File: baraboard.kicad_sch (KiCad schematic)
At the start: 27 parts, among them J1 OLED_128x64, U1 MCU_Seeed_XIAO_RP2040

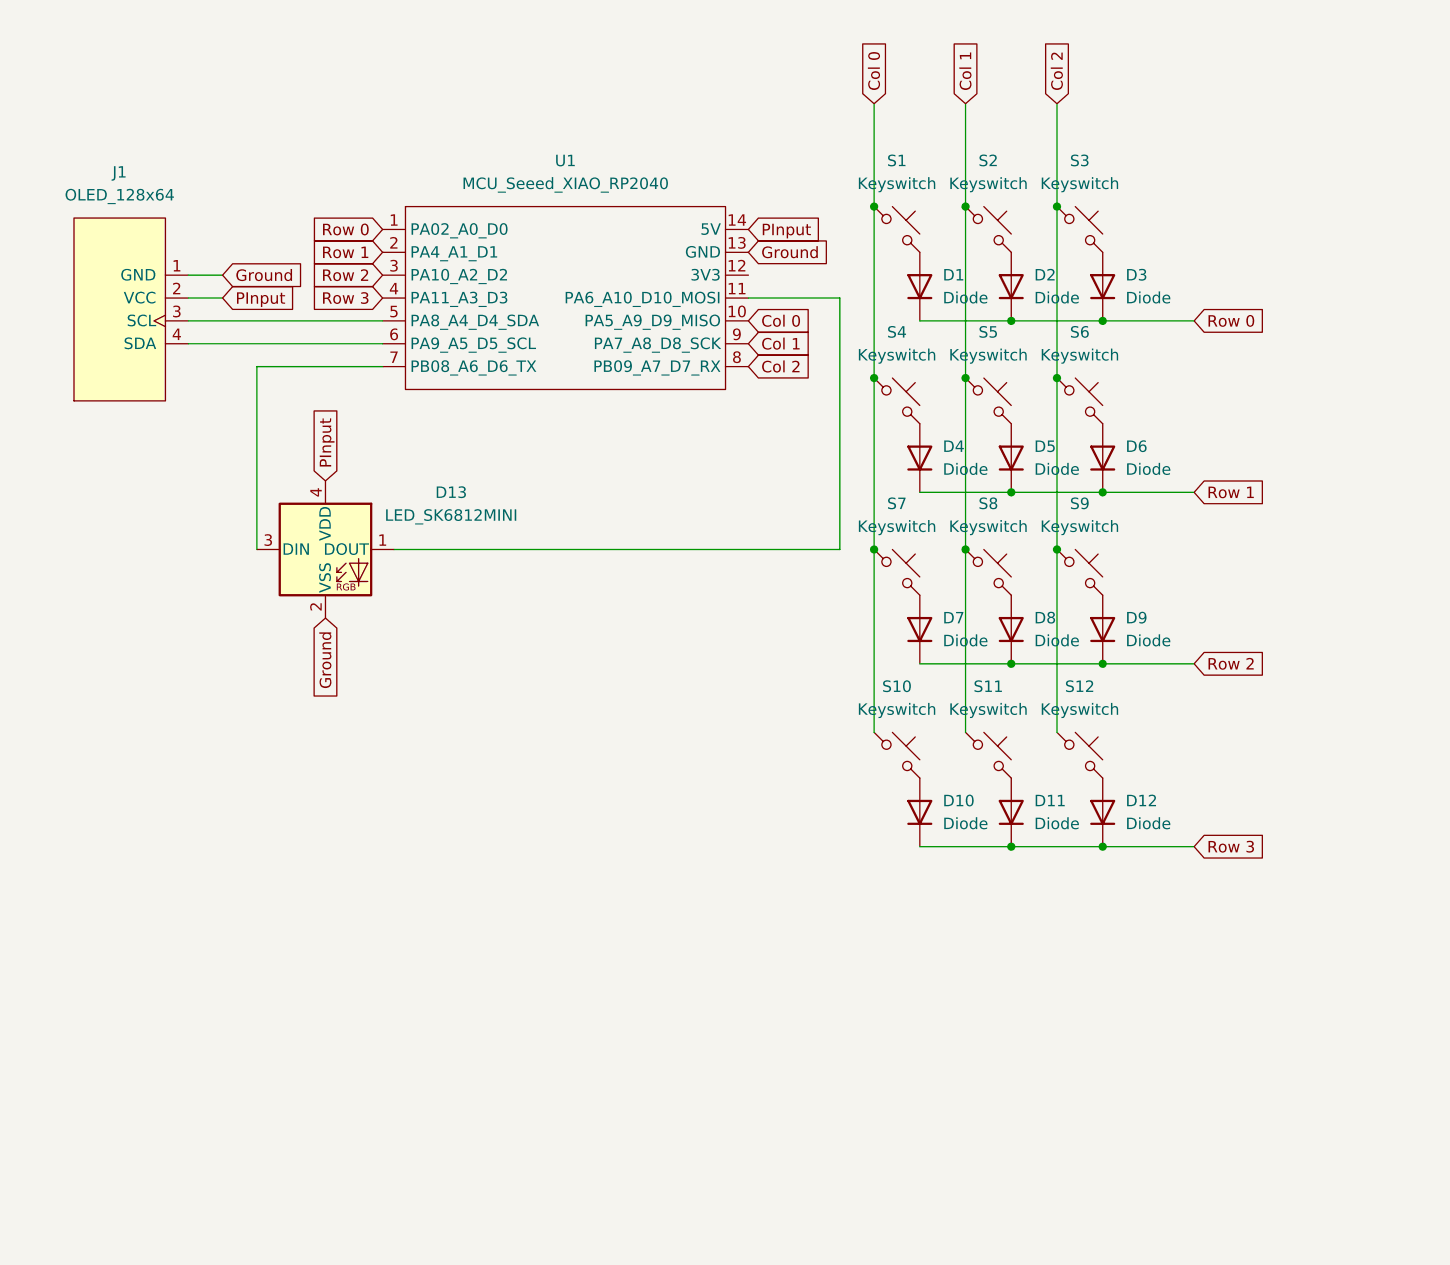
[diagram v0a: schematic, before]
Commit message: schema is done, pcb on the way
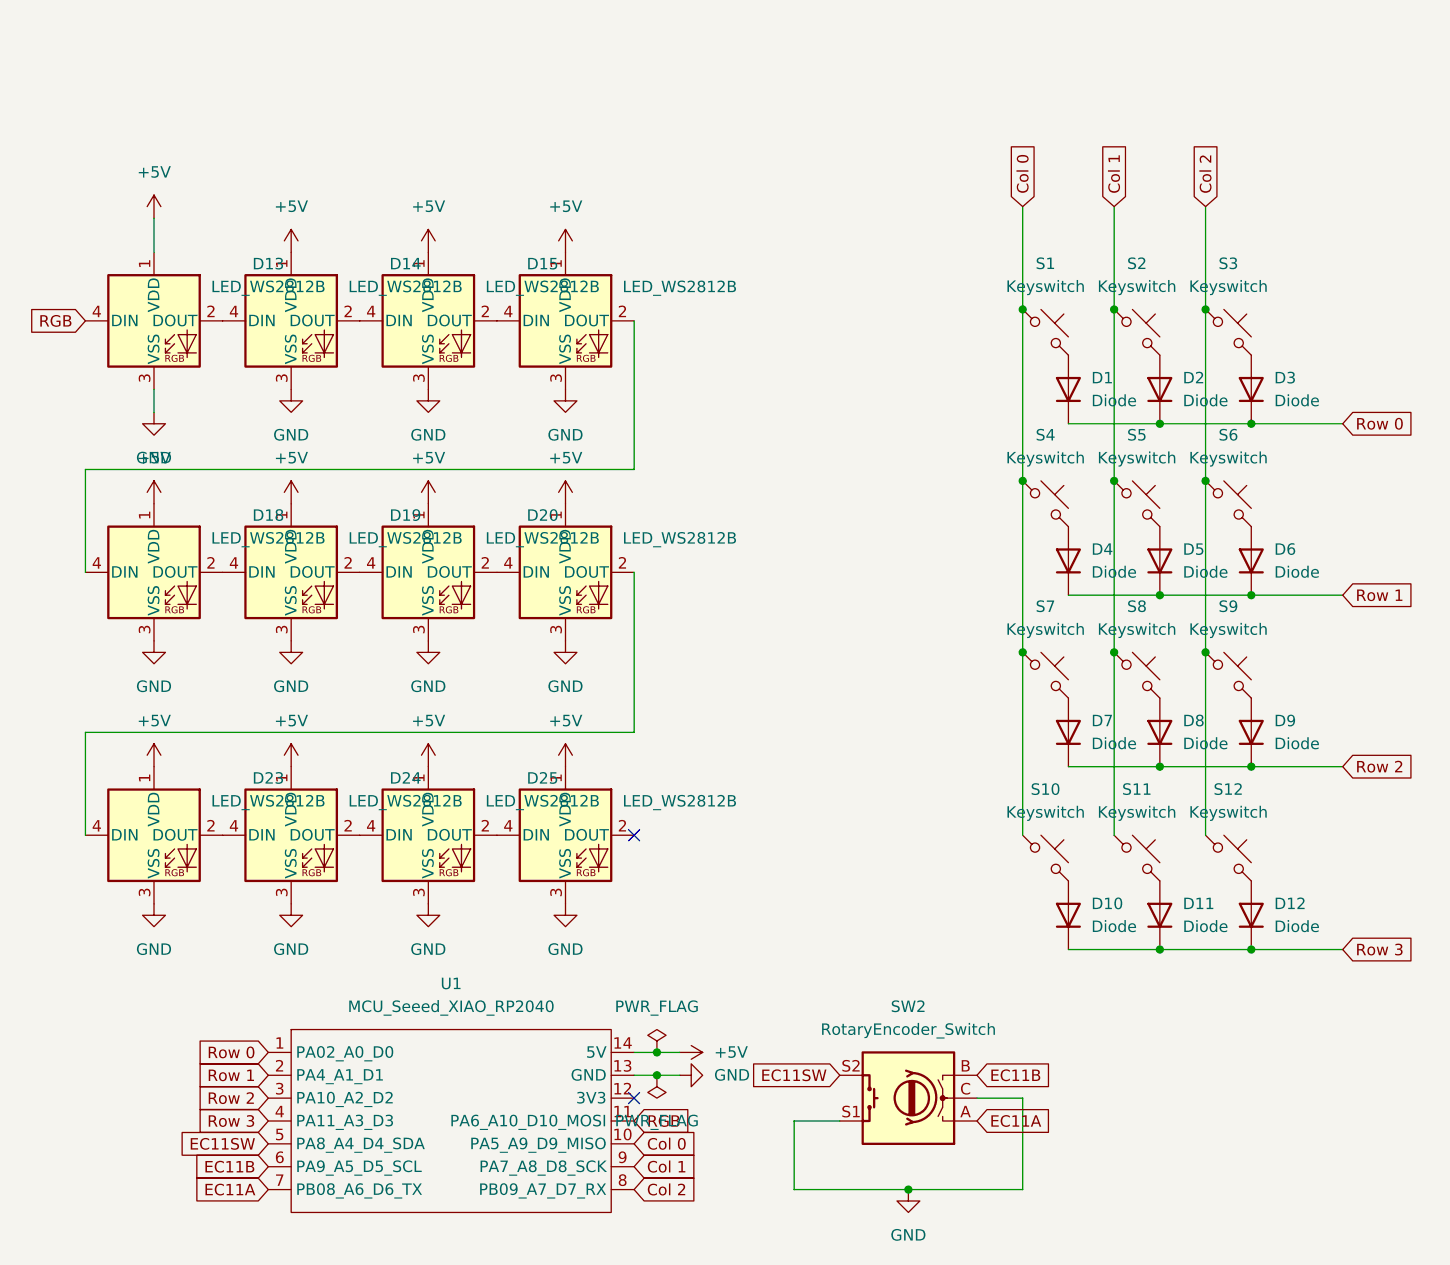
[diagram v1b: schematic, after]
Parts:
- removed D13: LED_SK6812MINI, ScottoKeebs_Components:LED_SK6812MINI, symbol ScottoKeebs:LED_SK6812MINI
- removed J1: OLED_128x64, ScottoKeebs_Components:OLED_128x64, symbol ScottoKeebs:OLED_128x64
- added D13, D14, D15, D16, D18, D19, D20, D21, D23, D24, D25, D26: LED_WS2812B, ScottoKeebs_Components:LED_SK6812MINI, symbol ScottoKeebs:LED_WS2812B
- added SW2: RotaryEncoder_Switch, Rotary_Encoder:RotaryEncoder_Alps_EC11E-Switch_Vertical_H20mm, symbol Device:RotaryEncoder_Switch
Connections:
- net RGB: now reaches U1.11 (PA6_A10_D10_MOSI)
- net RGB: now also D13.4 (DIN)
- net EC11A: now reaches U1.7 (PB08_A6_D6_TX)
- net EC11A: now also SW2.A
- net EC11SW: now reaches U1.5 (PA8_A4_D4_SDA)
- net EC11SW: now also SW2.S2
- net EC11B: now reaches U1.6 (PA9_A5_D5_SCL)
- net EC11B: now also SW2.B
- net Ground renamed GND
- net GND: now also D13.3 (VSS), D14.3 (VSS), D15.3 (VSS), D16.3 (VSS), D18.3 (VSS), D19.3 (VSS), D20.3 (VSS), D21.3 (VSS), D23.3 (VSS), D24.3 (VSS), D25.3 (VSS), D26.3 (VSS), SW2.C, SW2.S1
- net PInput renamed +5V
- net +5V: now also D13.1 (VDD), D14.1 (VDD), D15.1 (VDD), D16.1 (VDD), D18.1 (VDD), D19.1 (VDD), D20.1 (VDD), D21.1 (VDD), D23.1 (VDD), D24.1 (VDD), D25.1 (VDD), D26.1 (VDD)
- new net: D19.2 (DOUT), D20.4 (DIN)
- new net: D18.2 (DOUT), D19.4 (DIN)
- new net: D24.2 (DOUT), D25.4 (DIN)
- new net: D23.2 (DOUT), D24.4 (DIN)
- new net: D21.2 (DOUT), D23.4 (DIN)
- new net: D20.2 (DOUT), D21.4 (DIN)
- new net: D25.2 (DOUT), D26.4 (DIN)
- new net: D13.2 (DOUT), D14.4 (DIN)
- new net: D16.2 (DOUT), D18.4 (DIN)
- new net: D15.2 (DOUT), D16.4 (DIN)
- new net: D14.2 (DOUT), D15.4 (DIN)
- no-connect marks 0 -> 2
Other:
- moved on the sheet: D1, D10, D11, D12, D2, D3, D4, D5, D6, D7, D8, D9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
